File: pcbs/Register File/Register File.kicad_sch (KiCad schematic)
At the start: 0 parts

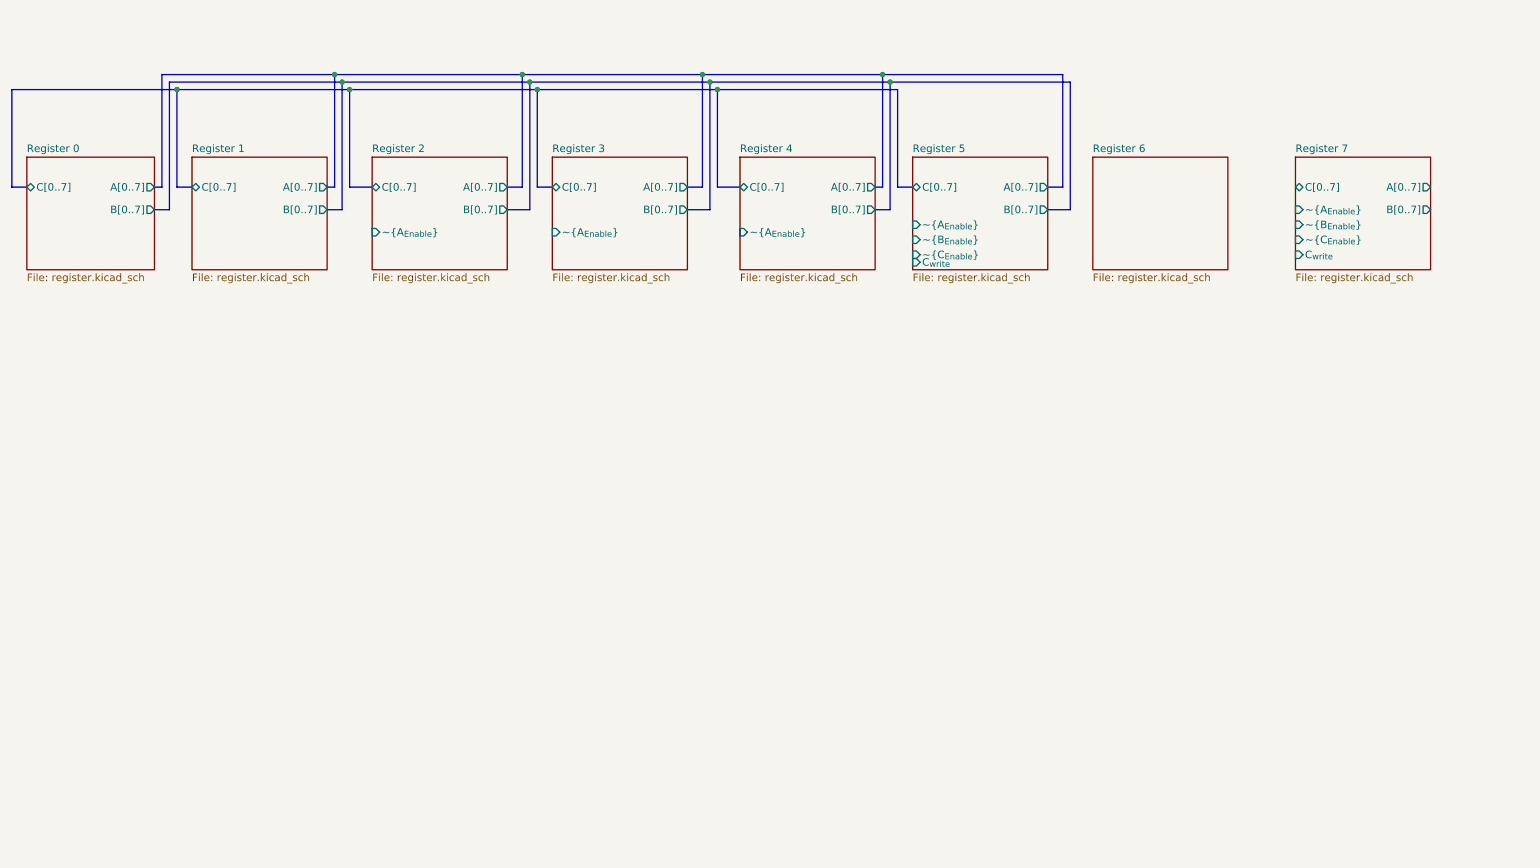
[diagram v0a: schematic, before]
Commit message: Yet more routing
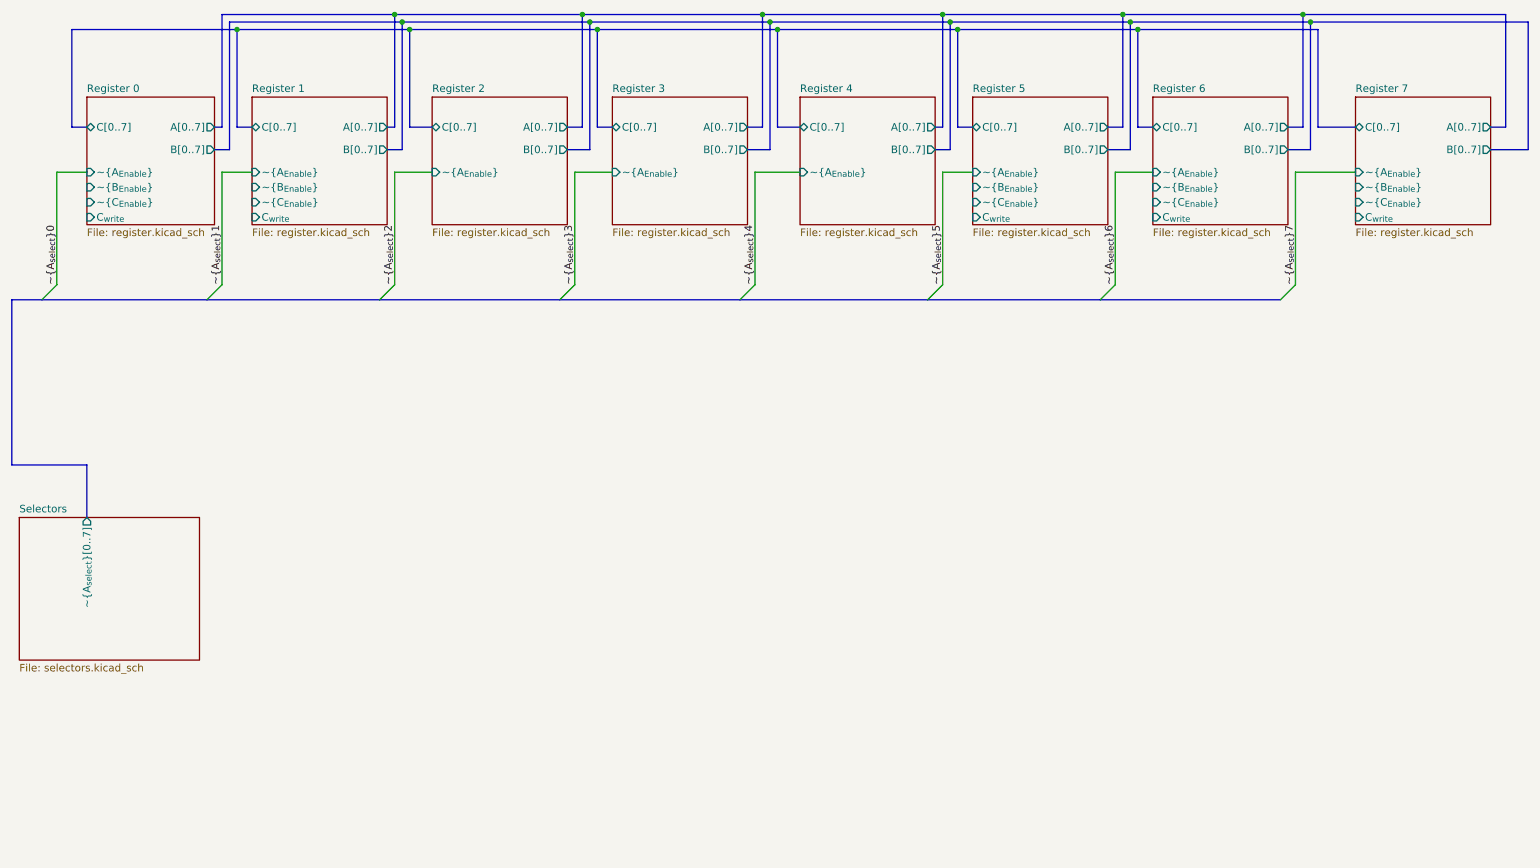
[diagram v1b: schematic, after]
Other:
- added sheet Selectors (selectors.kicad_sch)
- sheet Register 0 ports: added C_{write}, ~{A_{Enable}}, ~{B_{Enable}}, ~{C_{Enable}}; removed none
- sheet Register 1 ports: added C_{write}, ~{A_{Enable}}, ~{B_{Enable}}, ~{C_{Enable}}; removed none
- sheet Register 6 ports: added A[0..7], B[0..7], C[0..7], C_{write}, ~{A_{Enable}}, ~{B_{Enable}}, ~{C_{Enable}}; removed none

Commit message: More work
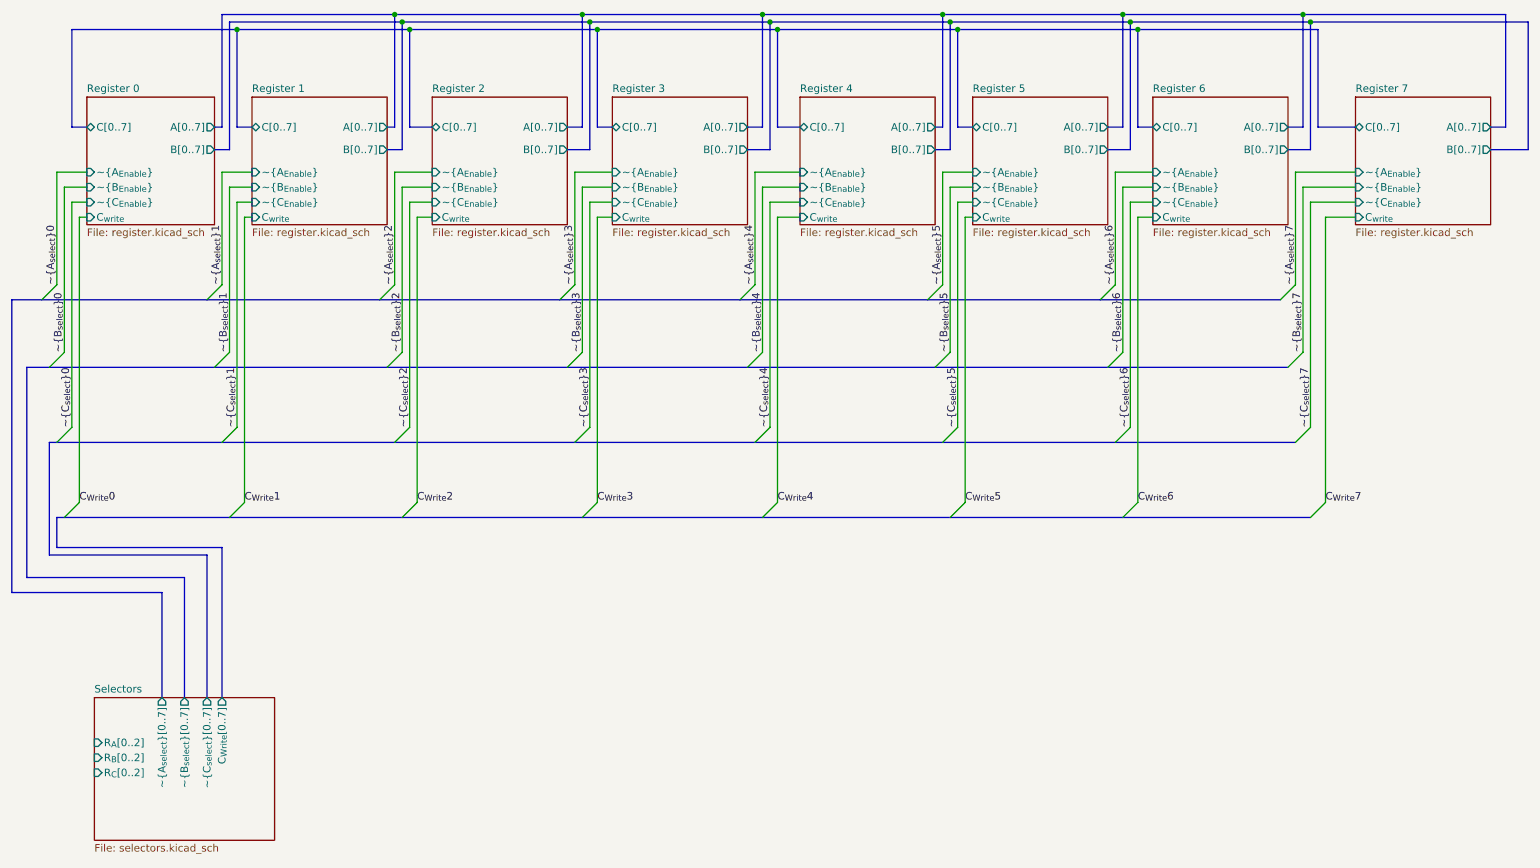
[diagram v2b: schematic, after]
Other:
- sheet Register 2 ports: added C_{write}, ~{B_{Enable}}, ~{C_{Enable}}; removed none
- sheet Register 3 ports: added C_{write}, ~{B_{Enable}}, ~{C_{Enable}}; removed none
- sheet Register 4 ports: added C_{write}, ~{B_{Enable}}, ~{C_{Enable}}; removed none
- sheet Selectors ports: added C_{Write}[0..7], R_{A}[0..2], R_{B}[0..2], R_{C}[0..2], ~{B_{select}}[0..7], ~{C_{select}}[0..7]; removed none
